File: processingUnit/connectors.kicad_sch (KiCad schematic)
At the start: 10 parts, among them J101 Conn_01x05, J102 Conn_01x04, J103 Conn_01x07, J104 Conn_01x10

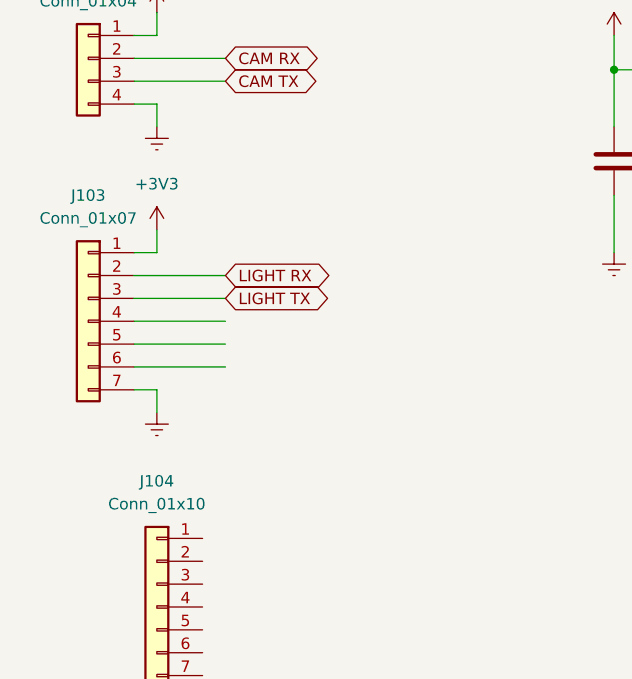
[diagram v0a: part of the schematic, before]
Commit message: L3 Schematic
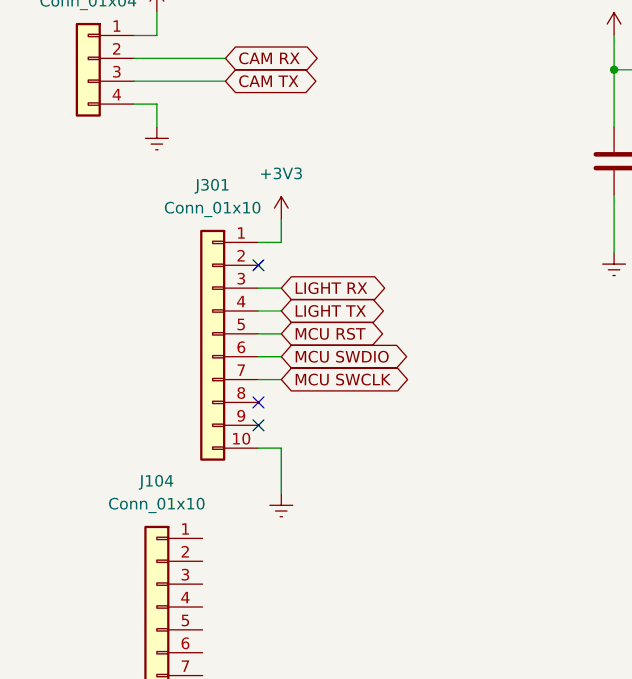
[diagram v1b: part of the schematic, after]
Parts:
- removed J103: Conn_01x07, Connector_JST:JST_XH_S7B-XH-A_1x07_P2.50mm_Horizontal, symbol Connector_Generic:Conn_01x07
- added J301: Conn_01x10, Library:526101071, symbol Connector_Generic:Conn_01x10
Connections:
- net +3V3: now also J301.1 (Pin_1)
- net GNDREF: now also J301.10 (Pin_10)
- net LIGHT RX: now also J301.3 (Pin_3)
- net LIGHT TX: now also J301.4 (Pin_4)
- new net MCU RST: J301.5 (Pin_5)
- new net MCU SWCLK: J301.7 (Pin_7)
- new net MCU SWDIO: J301.6 (Pin_6)
- no-connect marks 0 -> 3
